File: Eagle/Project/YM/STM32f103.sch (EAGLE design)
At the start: 70 parts, among them IC1 YM3812, IC10 LM358D, IC11 YM3014B, IC12 LM358D, IC13 YM3812, IC14 YM3014B, IC15 LM358D, IC3 BA033CC0T, IC4 LM2575-5.0S, IC5 YM3812, IC6 YM3014B, IC7 YM3014B, IC8 LM358D, IC9 YM3812, J1 DIN5, Q1 6N136SDM, U1 STM32F10XRXT6, U2 74AC04MTC, X1 CRYSTALS-NOGND-4-HSMX

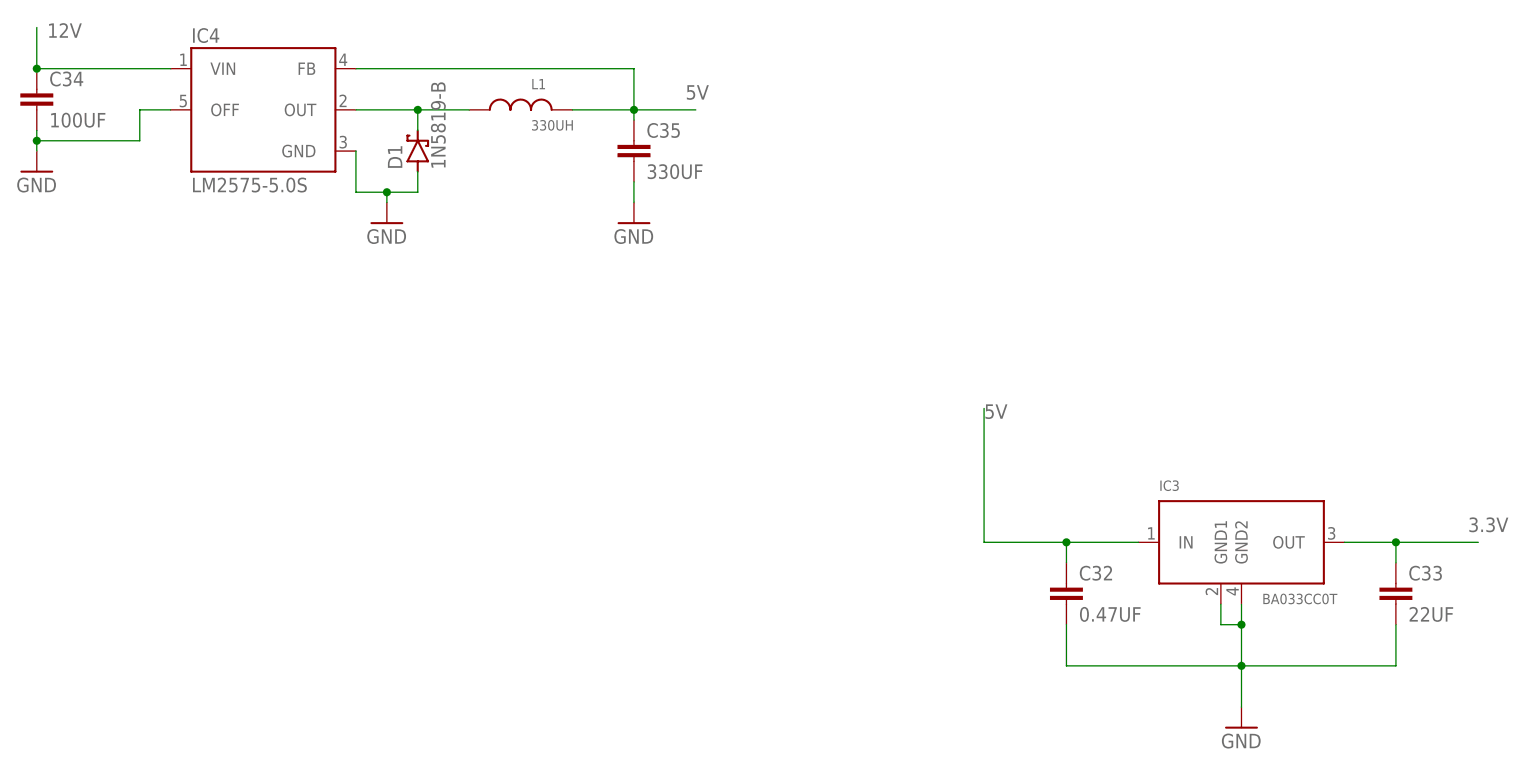
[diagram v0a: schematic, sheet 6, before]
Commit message: USB CONN
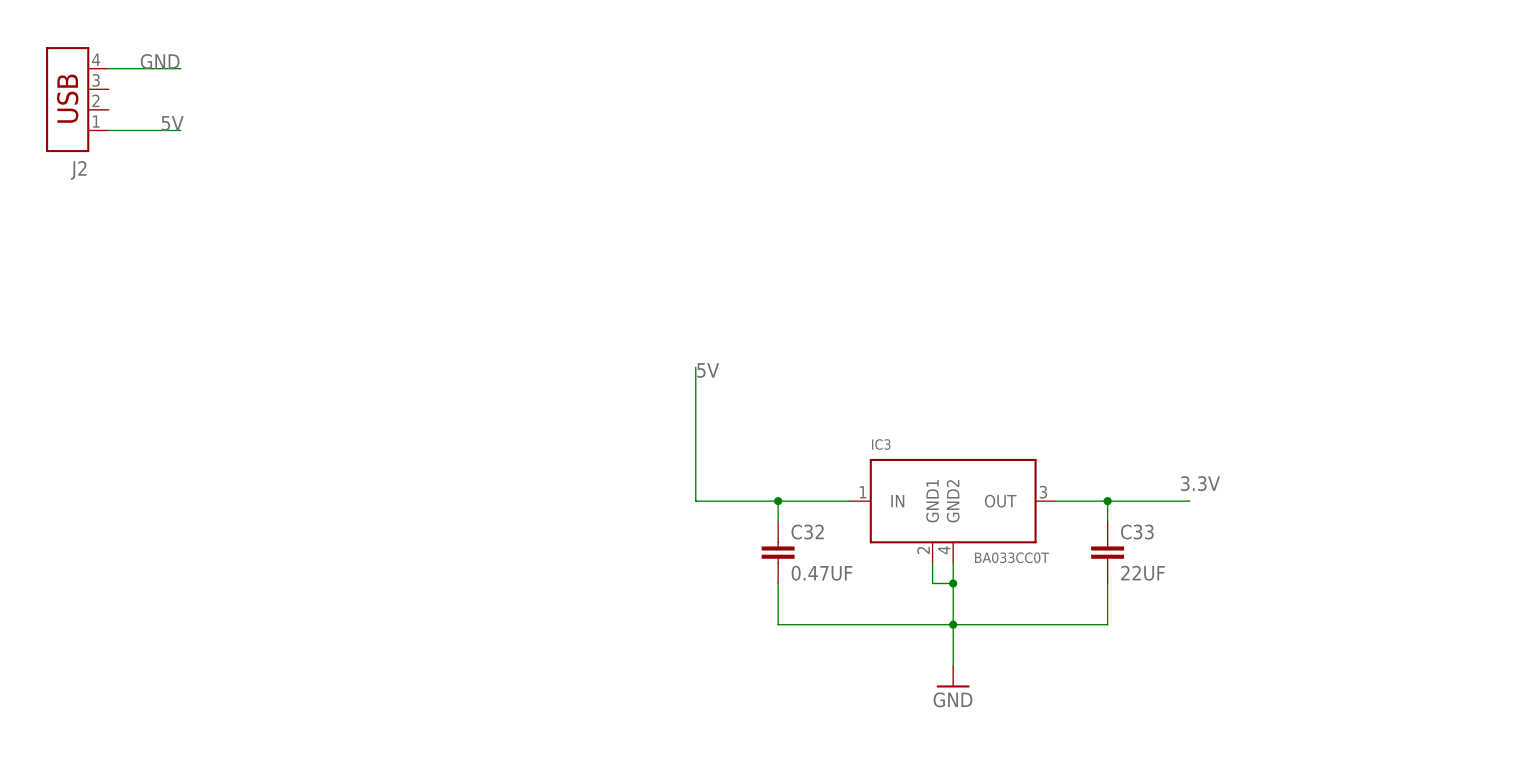
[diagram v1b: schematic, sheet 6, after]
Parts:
- removed C34: 100UF, +HU-Lib:100UF
- removed C35: 330UF, +HU-Lib:330UF
- removed D1: 1N5819-B, diode:1N5819-B
- removed IC4: LM2575-5.0S, lm2575:LM2575-5.0S
- removed L1: 330UH, +HU-Lib:330UH
- added J2: (no value), LDO:CON-USB-B
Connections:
- removed net 12V: C34.1, IC4.VIN
- removed net N$15: D1.C, IC4.OUT, L1.P$2
- net 5V: now also J2.1; no longer C35.1, IC4.FB, L1.P$1
- net GND: now also J2.4; no longer C34.2, C35.2, D1.A, IC4.GND, IC4.OFF
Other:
- moved on the sheet: C32, C33, IC3
